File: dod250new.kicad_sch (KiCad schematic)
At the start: 31 parts, among them J1 Barrel_Jack_Switch, J2 NRJ4HF-1, J3 NRJ4HF, SW1 SW_FSW800_3PDT, U1 TL071

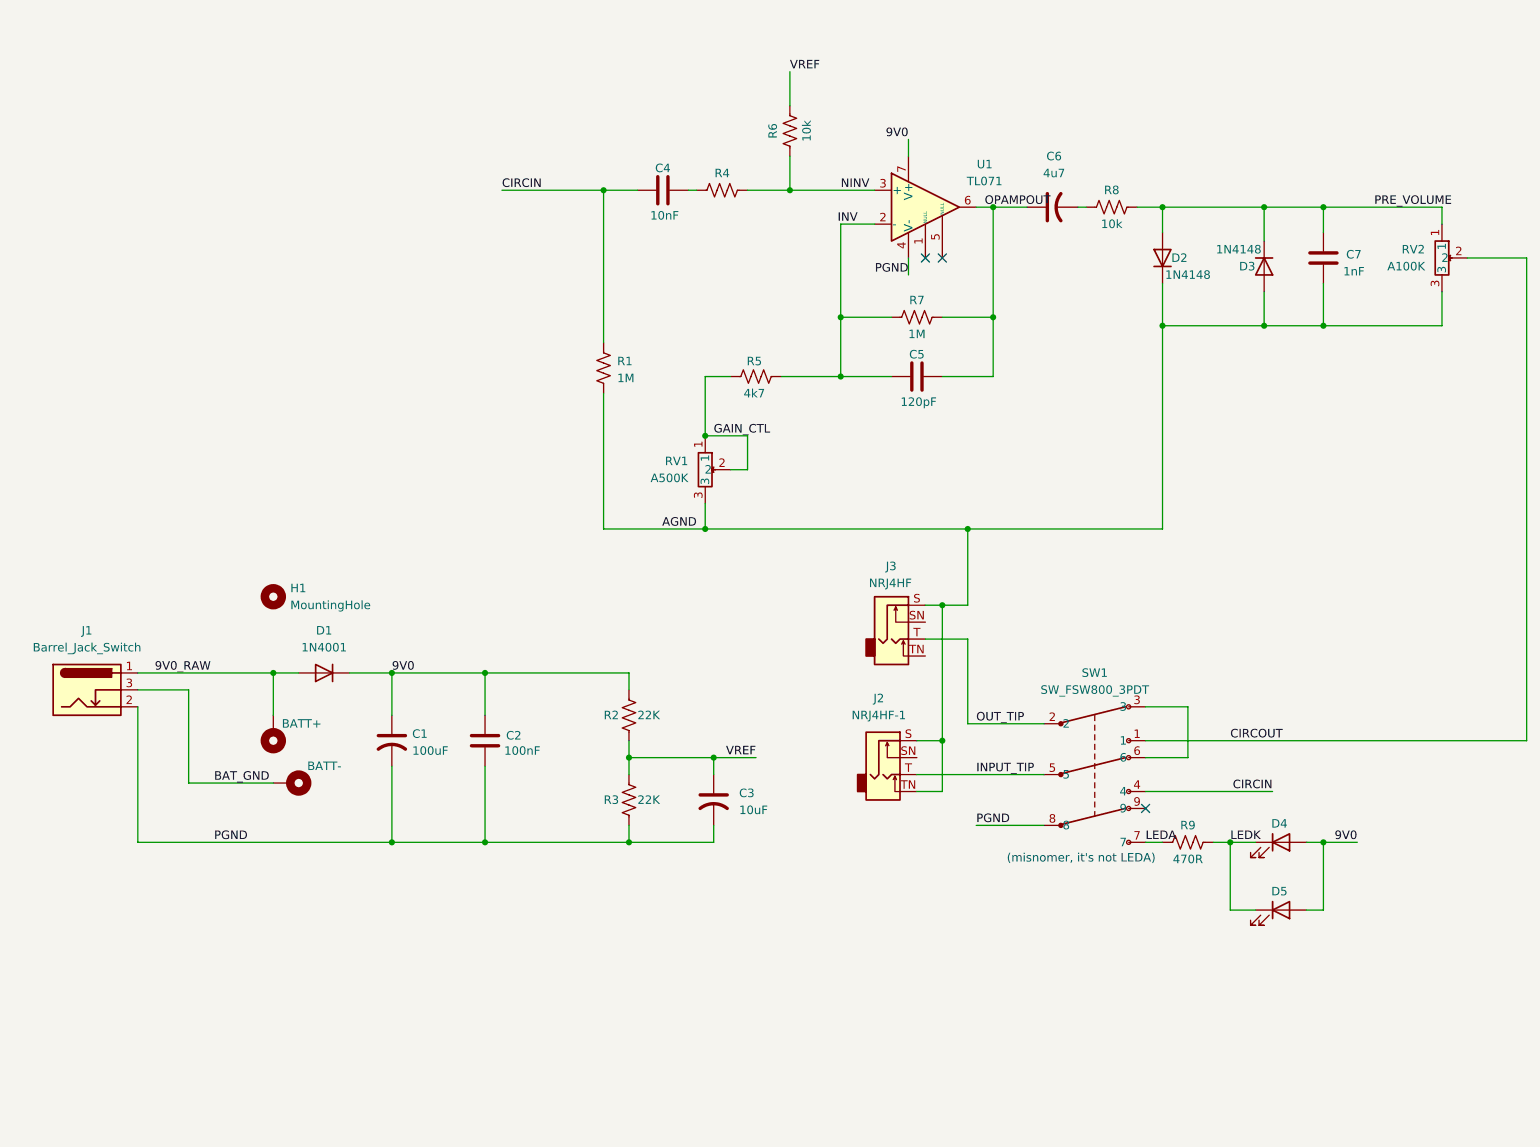
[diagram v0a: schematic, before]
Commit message: minor tweaks
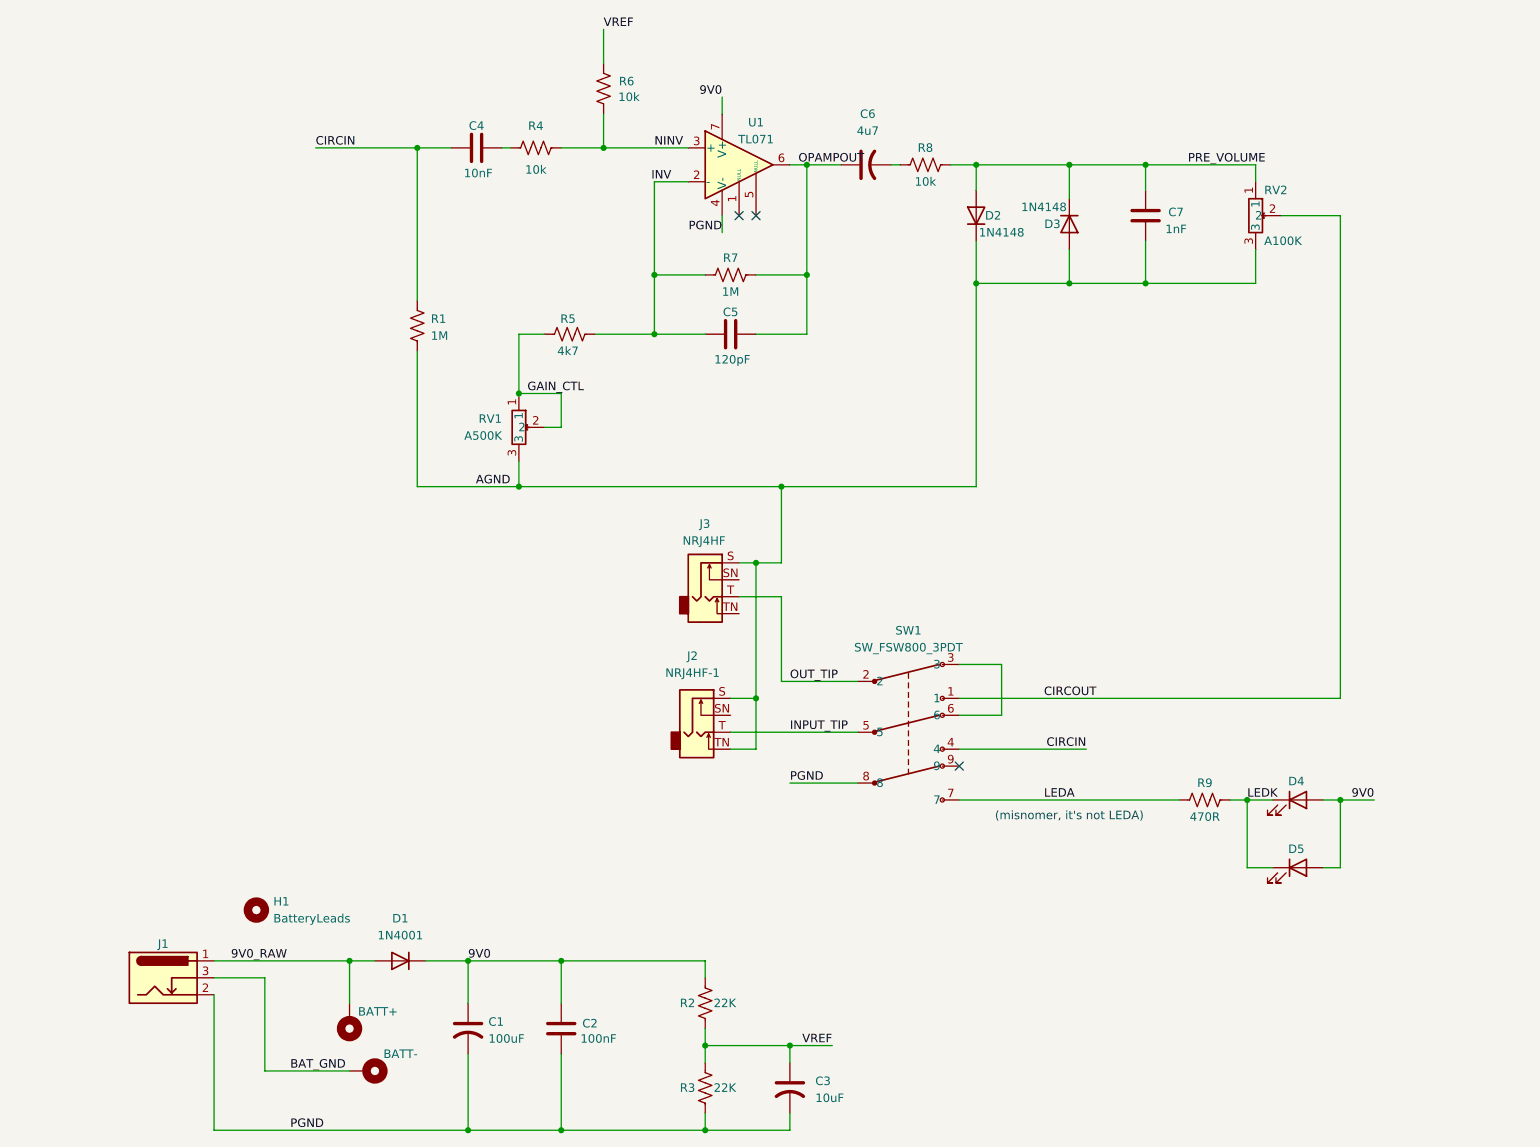
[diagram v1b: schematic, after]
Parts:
- H1: value MountingHole -> BatteryLeads
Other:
- company: github.com/whbeers/buffer_overflow -> dod250.shupac.com/v1_1
- title: Buffer Overflow Drive Effect -> DOD Overdrive Preamp 250
- moved on the sheet: C1, C2, C3, C4, C5, C6, C7, D1, D2, D3, D4, D5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
